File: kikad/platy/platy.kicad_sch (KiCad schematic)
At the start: 31 parts, among them U1 ESP32-S3, U2 APS6404L-3SQRx-SN, U3 W25Q128JVS, U4 CC1101, Y1 40Mhz(+-10 ppm), Y2 Crystal

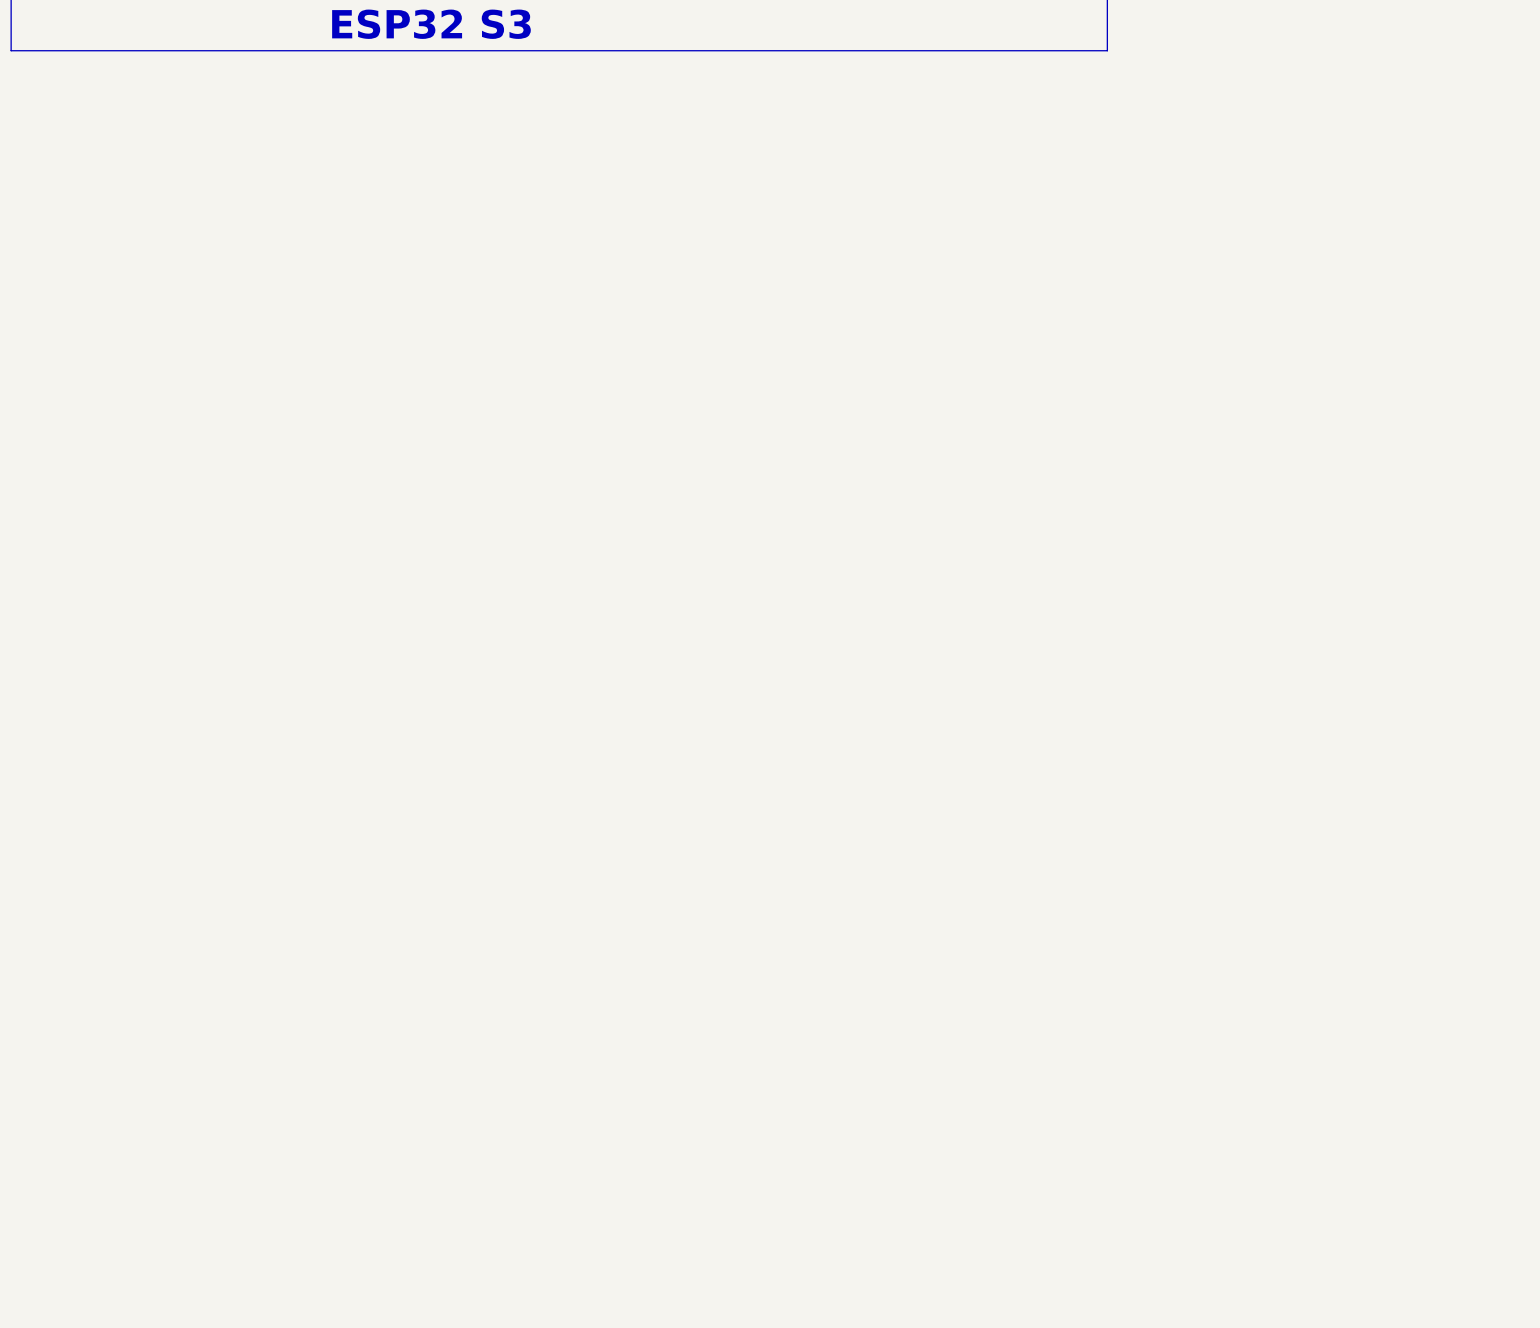
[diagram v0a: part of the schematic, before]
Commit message: Updated the schiematic
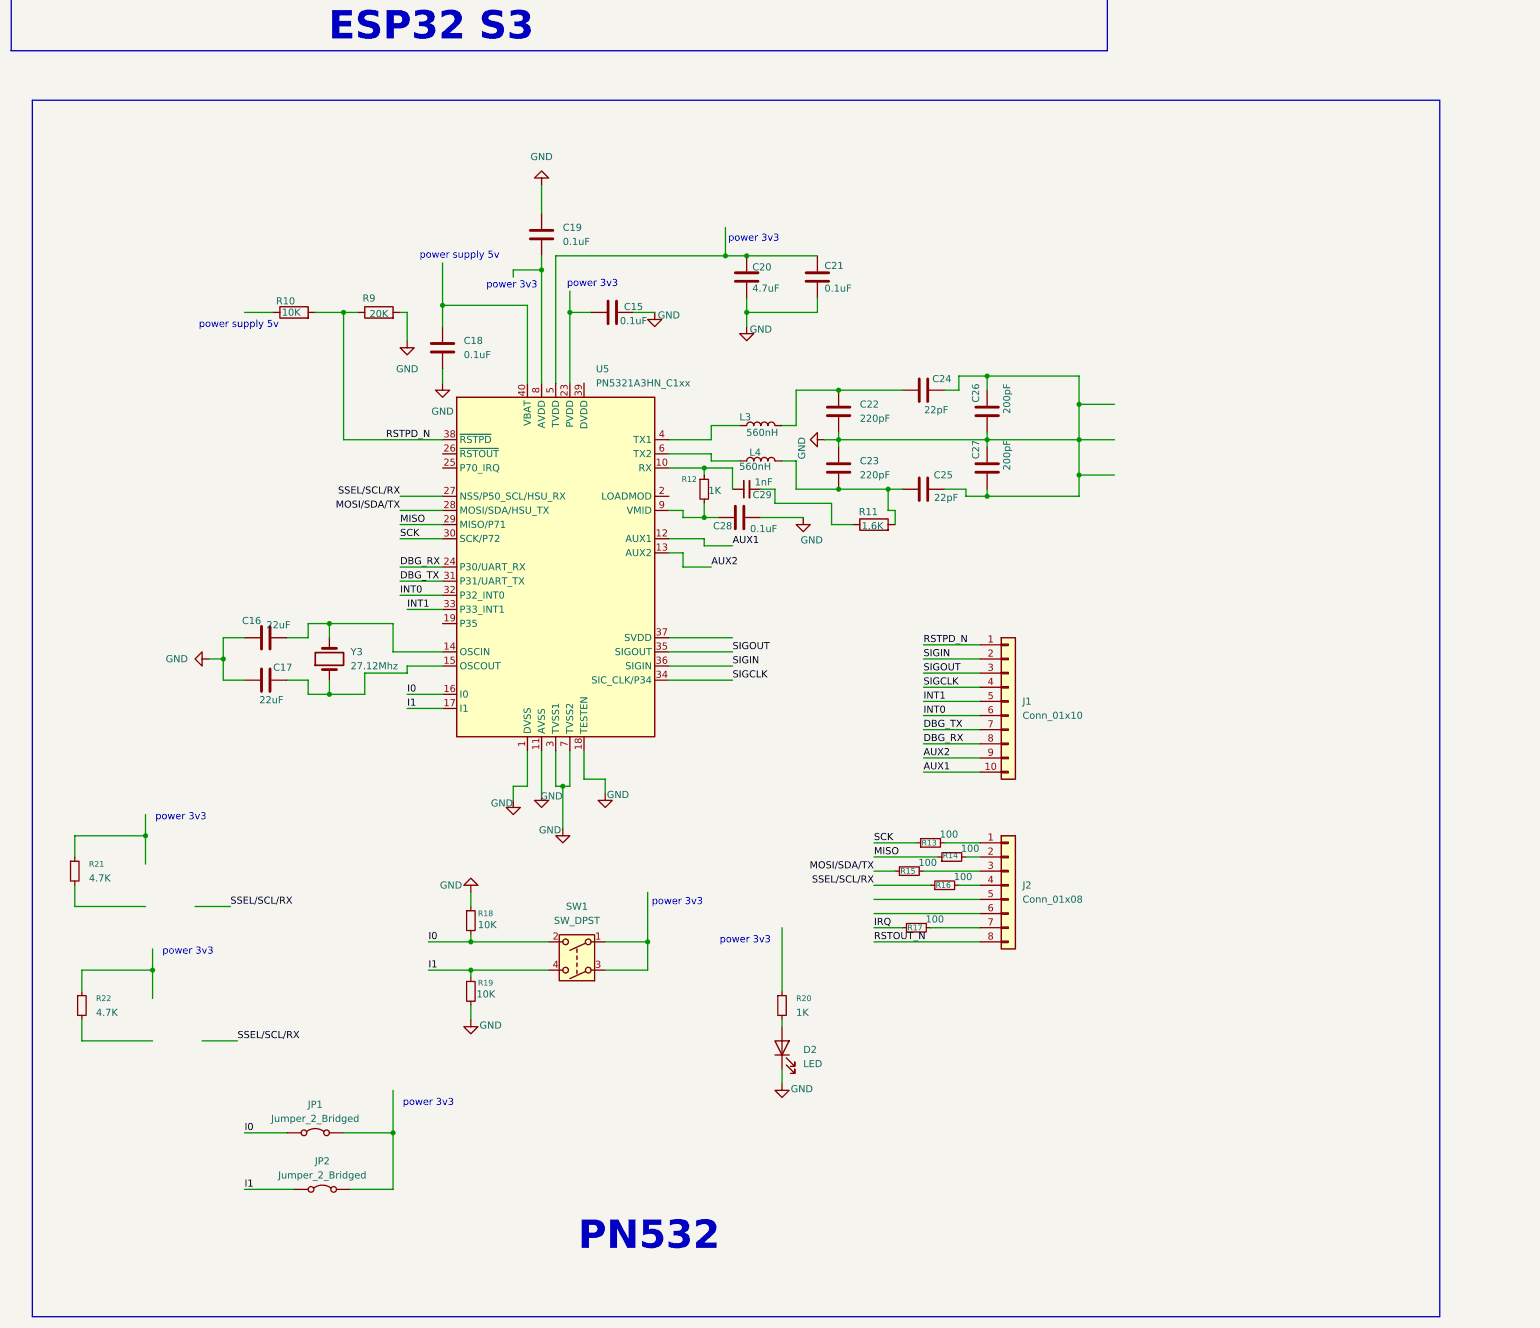
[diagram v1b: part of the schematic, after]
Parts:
- added C15, C18, C19, C21, C28: 0.1uF, symbol Device:C
- added C16, C17: 22uF, symbol Device:C
- added C20: 4.7uF, symbol Device:C
- added C22, C23: 220pF, symbol Device:C
- added C24, C25: 22pF, symbol Device:C
- added C26, C27: 200pF, symbol Device:C
- added C29: 1nF, symbol Device:C_Small
- added D2: LED, symbol Device:LED
- added J1: Conn_01x10, symbol Connector_Generic:Conn_01x10
- added J2: Conn_01x08, symbol Connector_Generic:Conn_01x08
- added JP1, JP2: Jumper_2_Bridged, symbol Jumper:Jumper_2_Bridged
- added L3, L4: 560nH, symbol Device:L
- added R10: 10K, symbol Device:R
- added R11: 1.6K, symbol Device:R
- added R12, R20: 1K, symbol Device:R_Small
- added R13, R14, R15, R16, R17: 100, symbol Device:R_Small
- added R18, R19: 10K, symbol Device:R_Small
- added R21, R22: 4.7K, symbol Device:R_Small
- added R9: 20K, symbol Device:R
- added SW1: SW_DPST, symbol Switch:SW_DPST
- added U5: PN5321A3HN_C1xx, Package_DFN_QFN:HVQFN-40-1EP_6x6mm_P0.5mm_EP4.1x4.1mm, symbol RF_NFC:PN5321A3HN_C1xx
- added Y3: 27.12Mhz, symbol Device:Crystal
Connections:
- net GND: now also C15.2, C16.2, C17.1, C18.2, C19.1, C20.2, C21.2, C22.2, C23.1, C24.2, C25.2, C26.1, C26.2, C27.1, C27.2, C28.2, D2.1 (K), R18.1, R19.2, R9.2, U5.1 (DVSS), U5.11 (AVSS), U5.18 (TESTEN), U5.3 (TVSS1), U5.41 (AVSS), U5.7 (TVSS2)
- new net: J2.2 (Pin_2), R14.2
- new net: C16.1, U5.14 (OSCIN), Y3.2
- new net: L4.1, U5.6 (TX2)
- new net: C23.2, C25.1, L4.2, R11.2
- new net: J2.1 (Pin_1), R13.2
- new net: J2.3 (Pin_3), R15.2
- new net: J2.4 (Pin_4), R16.2
- new net: J2.7 (Pin_7), R17.2
- new net: C29.1, R12.1, U5.10 (RX)
- new net: C17.2, U5.15 (OSCOUT), Y3.1
- new net: C15.1, U5.23 (PVDD)
- new net: L3.1, U5.4 (TX1)
- new net: C18.1, U5.40 (VBAT)
- new net: C20.1, C21.1, U5.5 (TVDD)
- new net: C19.2, U5.8 (AVDD)
- new net: C28.1, R12.2, U5.9 (VMID)
- new net: C22.1, C24.1, L3.2
- new net: C29.2, R11.1
- new net: D2.2 (A), R20.2
- new net: JP1.2 (B), JP2.2 (B)
- new net: SW1.1, SW1.3
- new net AUX1: J1.10 (Pin_10), U5.12 (AUX1)
- new net AUX2: J1.9 (Pin_9), U5.13 (AUX2)
- new net DBG_RX: J1.8 (Pin_8), U5.24 (P30/UART_RX)
- new net DBG_TX: J1.7 (Pin_7), U5.31 (P31/UART_TX)
- new net I0: JP1.1 (A), R18.2, SW1.2, U5.16 (I0)
- new net I1: JP2.1 (A), R19.1, SW1.4, U5.17 (I1)
- new net INT0: J1.6 (Pin_6), U5.32 (P32_INT0)
- new net INT1: J1.5 (Pin_5), U5.33 (P33_INT1)
- new net IRQ: R17.1
- new net MISO: R14.1, U5.29 (MISO/P71)
- new net MOSI/SDA/TX: R15.1, U5.28 (MOSI/SDA/HSU_TX)
- new net RSTOUT_N: J2.8 (Pin_8)
- new net RSTPD_N: J1.1 (Pin_1), R10.2, R9.1, U5.38 (~{RSTPD})
- new net SCK: R13.1, U5.30 (SCK/P72)
- new net SIGCLK: J1.4 (Pin_4), U5.34 (SIC_CLK/P34)
- new net SIGIN: J1.2 (Pin_2), U5.36 (SIGIN)
- new net SIGOUT: J1.3 (Pin_3), U5.35 (SIGOUT)
- new net SSEL/SCL/RX: R16.1, U5.27 (NSS/P50_SCL/HSU_RX)
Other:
- note added: "PN532"
- note added: "power 3v3"
- note added: "power supply 5v"
